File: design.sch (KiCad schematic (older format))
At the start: 6 parts, among them J1 USB_C_Receptacle, J2 Conn_01x05, U1 ATtiny1616-M

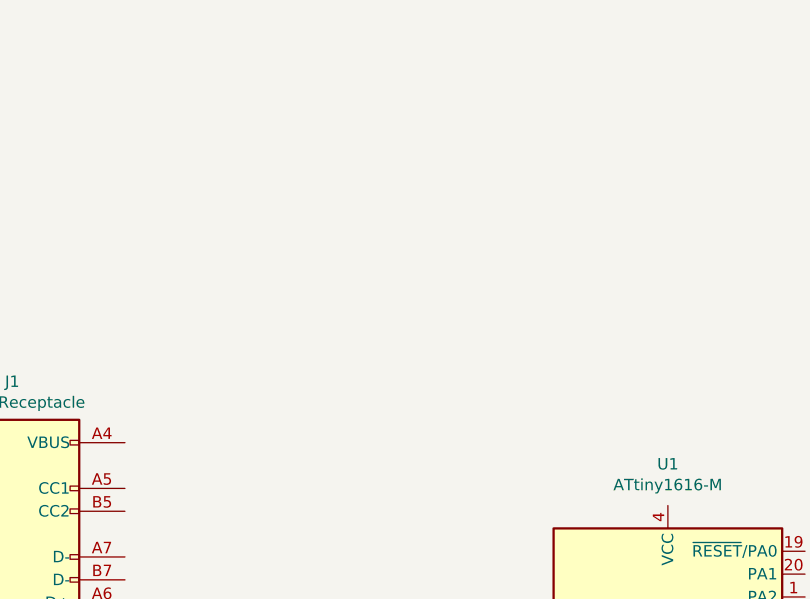
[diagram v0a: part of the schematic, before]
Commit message: test
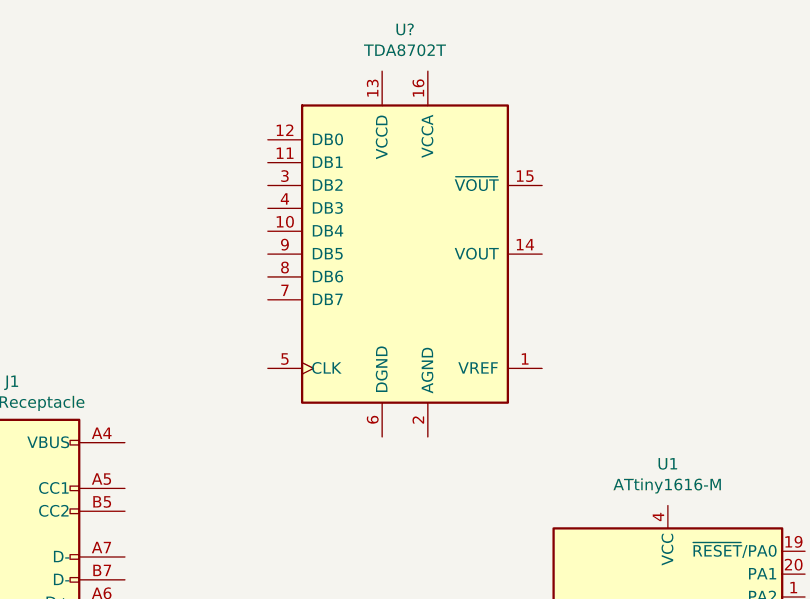
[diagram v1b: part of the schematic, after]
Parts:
- added U?: TDA8702T, symbol Video:TDA8702T
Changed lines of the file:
@@
+	1    0    0    -1
+$EndComp
+$Comp
+L Video:TDA8702T U?
+U 1 1 6174D894
+P 4500 1750
+F 0 "U?" H 4500 2731 50  0000 C CNN
+F 1 "TDA8702T" H 4500 2640 50  0000 C CNN
+F 2 "" H 4500 1650 50  0001 C CIN
+F 3 "philips/tda8702.pdf" H 4500 1650 50  0001 C CNN
+	1    4500 1750
 	1    0    0    -1
 $EndComp

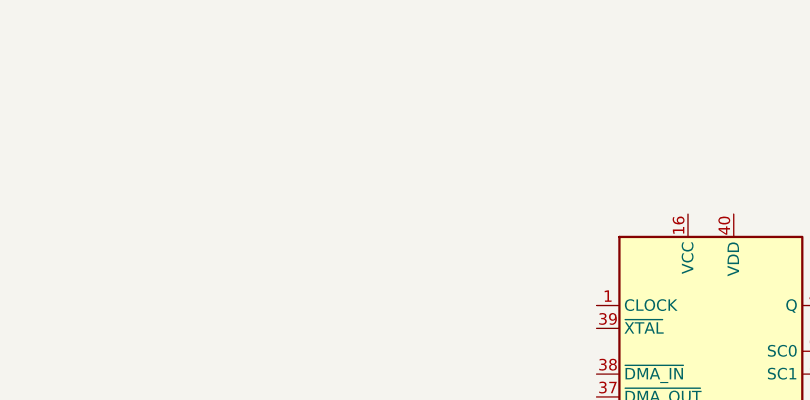
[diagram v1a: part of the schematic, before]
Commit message: test
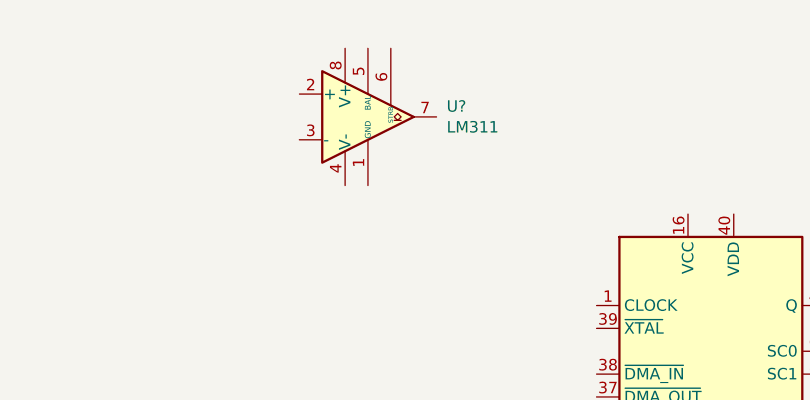
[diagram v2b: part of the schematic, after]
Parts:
- added U?: LM311, symbol Comparator:LM311
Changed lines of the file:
@@
+	1    0    0    -1
+$EndComp
+$Comp
+L Comparator:LM311 U?
+U 1 1 6174E38B
+P 7900 1150
+F 0 "U?" H 8244 1196 50  0000 L CNN
+F 1 "LM311" H 8244 1105 50  0000 L CNN
+F 2 "" H 7900 1150 50  0001 C CNN
+F 3 "https://www.st.com/resource/en/datasheet/lm311.pdf" H 7900 1150 50  0001 C CNN
+	1    7900 1150
 	1    0    0    -1
 $EndComp

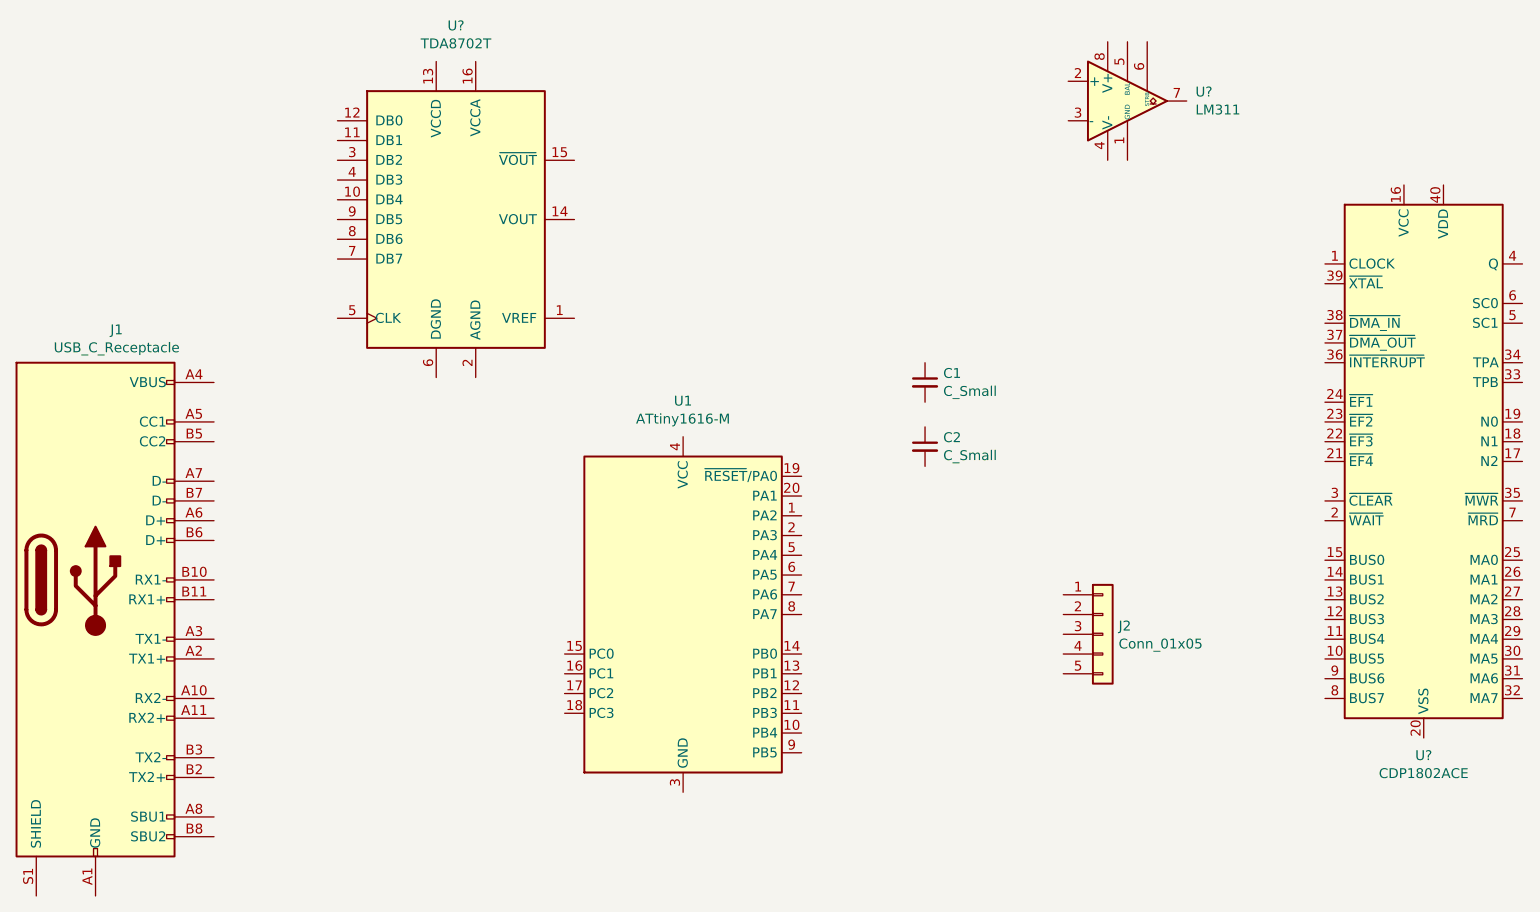
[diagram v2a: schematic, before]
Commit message: remove test components
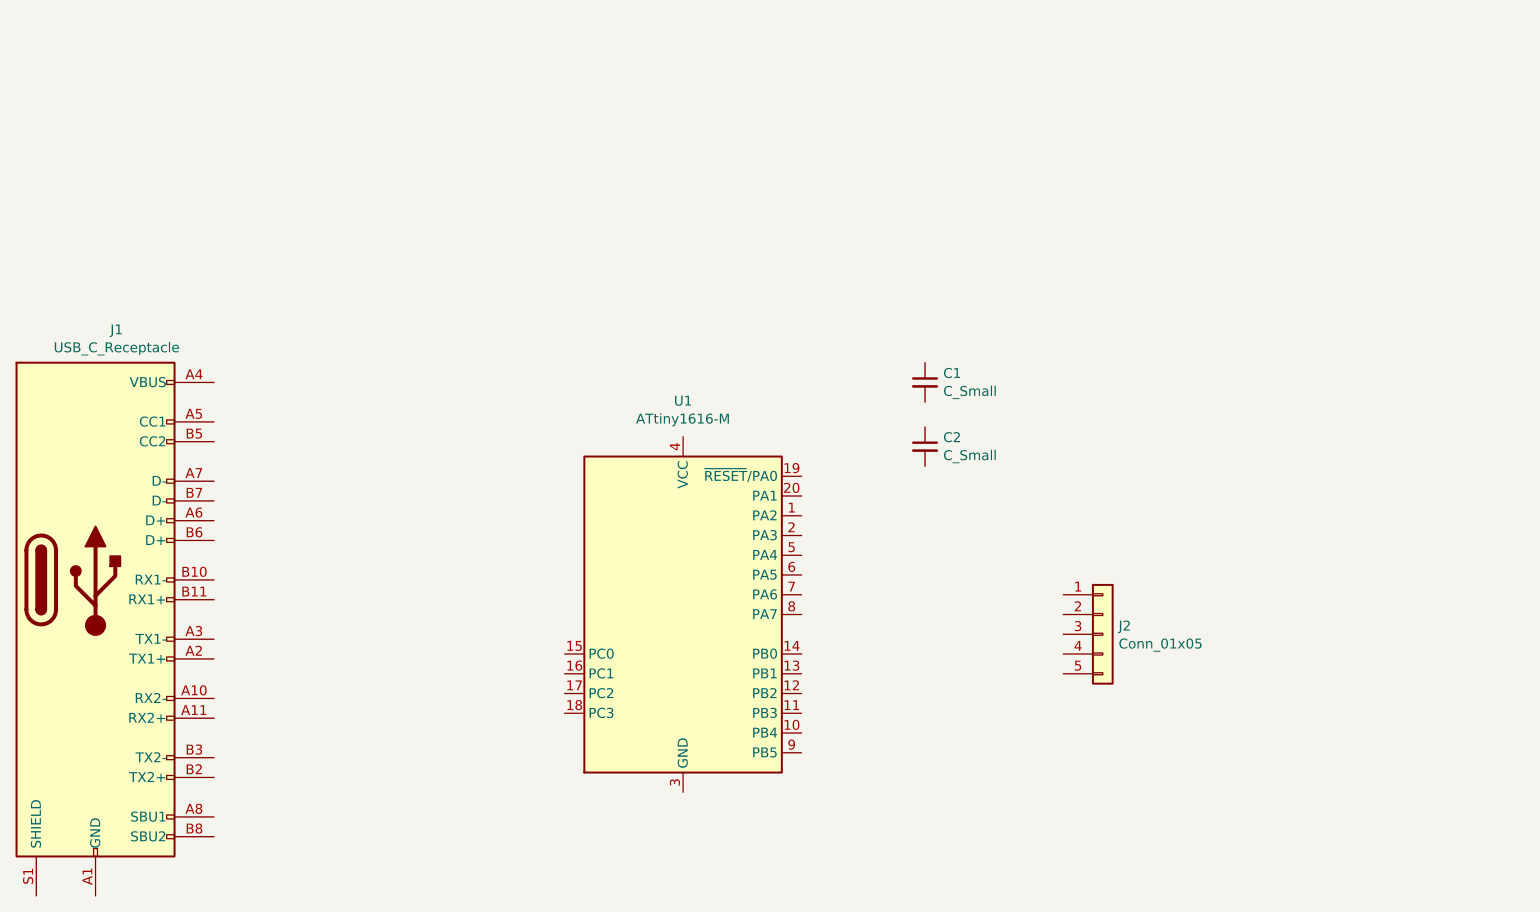
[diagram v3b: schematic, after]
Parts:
- removed U?: CDP1802ACE, Package_DIP:DIP-40_W15.24mm, symbol CPU:CDP1802ACE
- removed U?: TDA8702T, symbol Video:TDA8702T
- removed U?: LM311, symbol Comparator:LM311
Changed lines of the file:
@@
-	1    0    0    -1
-$EndComp
-$Comp
-L CPU:CDP1802ACE U?
-U 1 1 6174CECA
-P 9400 2975
-F 0 "U?" H 9400 1486 50  0000 C CNN
-F 1 "CDP1802ACE" H 9400 1395 50  0000 C CNN
-F 2 "Package_DIP:DIP-40_W15.24mm" H 9400 4875 50  0001 C CNN
-F 3 "http://www.cosmacelf.com/publications/data-sheets/cdp1802.pdf" H 9400 4975 50  0001 C CNN
-	1    9400 2975
-	1    0    0    -1
-$EndComp
-$Comp
-L Video:TDA8702T U?
-U 1 1 6174D894
-P 4500 1750
-F 0 "U?" H 4500 2731 50  0000 C CNN
-F 1 "TDA8702T" H 4500 2640 50  0000 C CNN
-F 2 "" H 4500 1650 50  0001 C CIN
-F 3 "philips/tda8702.pdf" H 4500 1650 50  0001 C CNN
-	1    4500 1750
-	1    0    0    -1
-$EndComp
-$Comp
-L Comparator:LM311 U?
-U 1 1 6174E38B
-P 7900 1150
-F 0 "U?" H 8244 1196 50  0000 L CNN
-F 1 "LM311" H 8244 1105 50  0000 L CNN
-F 2 "" H 7900 1150 50  0001 C CNN
-F 3 "https://www.st.com/resource/en/datasheet/lm311.pdf" H 7900 1150 50  0001 C CNN
-	1    7900 1150
 	1    0    0    -1
 $EndComp

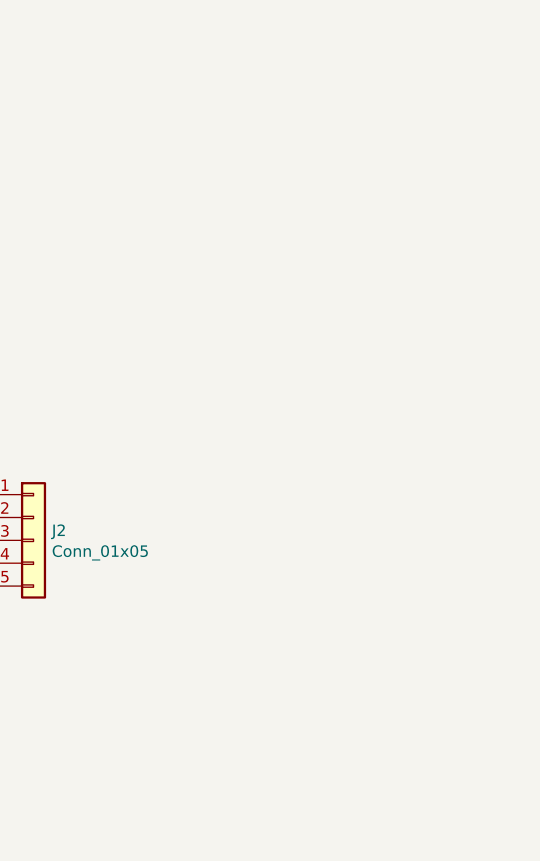
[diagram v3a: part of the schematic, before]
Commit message: test
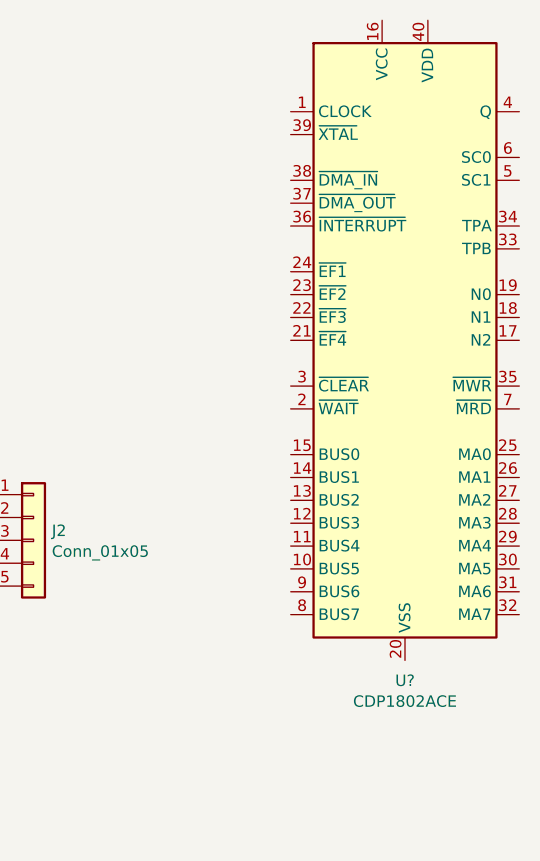
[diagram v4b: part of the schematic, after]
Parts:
- added U?: CDP1802ACE, Package_DIP:DIP-40_W15.24mm, symbol CPU:CDP1802ACE
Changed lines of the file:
@@
+	1    0    0    -1
+$EndComp
+$Comp
+L CPU:CDP1802ACE U?
+U 1 1 6174CECA
+P 9400 2975
+F 0 "U?" H 9400 1486 50  0000 C CNN
+F 1 "CDP1802ACE" H 9400 1395 50  0000 C CNN
+F 2 "Package_DIP:DIP-40_W15.24mm" H 9400 4875 50  0001 C CNN
+F 3 "http://www.cosmacelf.com/publications/data-sheets/cdp1802.pdf" H 9400 4975 50  0001 C CNN
+	1    9400 2975
 	1    0    0    -1
 $EndComp
